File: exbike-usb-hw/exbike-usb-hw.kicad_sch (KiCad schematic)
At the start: 19 parts, among them J1 ICSP, J2 USB_B, J3 AudioJack3_SwitchTR, J4 J1, J5 J2, U1 ATtiny24A-SS, U2 AMS1117-3.3, Y1 12 MHz

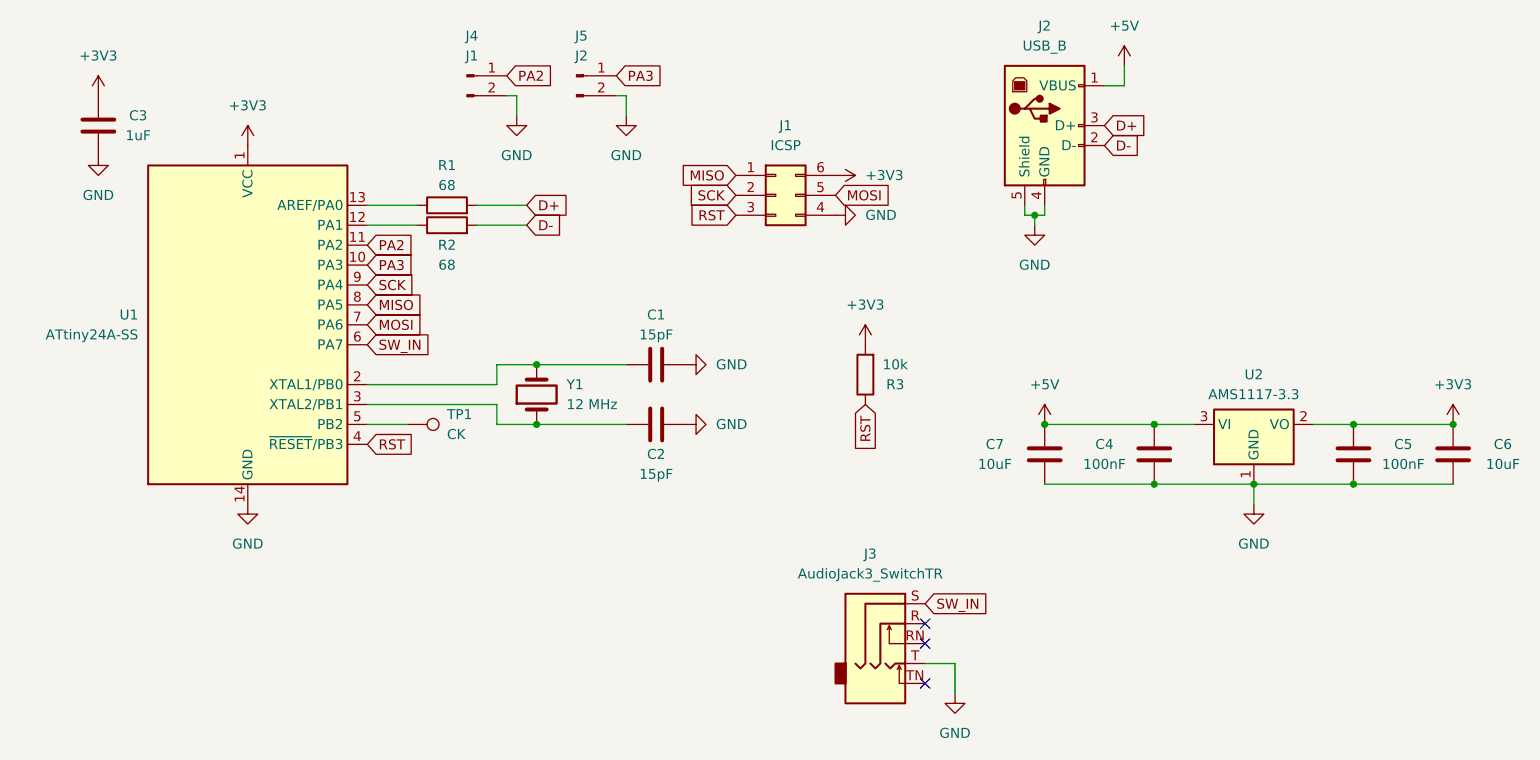
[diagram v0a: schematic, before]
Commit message: Layout
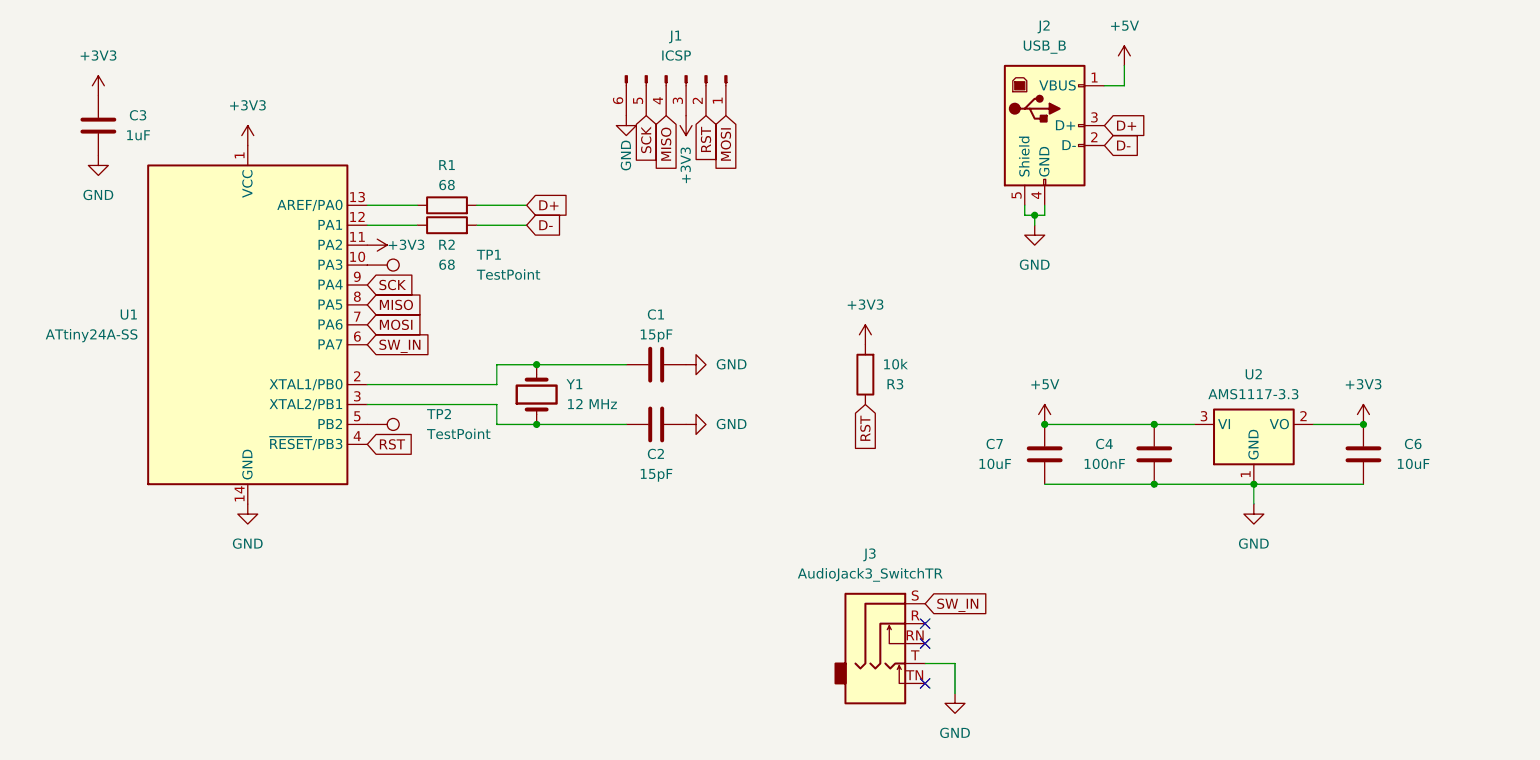
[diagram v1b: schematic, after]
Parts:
- removed C5: 100nF, Capacitor_SMD:C_0805_2012Metric_Pad1.18x1.45mm_HandSolder, symbol Device:C
- removed J1: ICSP, Connector_PinHeader_2.54mm:PinHeader_1x06_P2.54mm_Vertical, symbol Connector_Generic:Conn_02x03_Counter_Clockwise
- removed J4: J1, Connector_PinHeader_2.54mm:PinHeader_1x02_P2.54mm_Vertical, symbol Connector:Conn_01x02_Pin
- removed J5: J2, Connector_PinHeader_2.54mm:PinHeader_1x02_P2.54mm_Vertical, symbol Connector:Conn_01x02_Pin
- added J1: ICSP, Connector_PinHeader_2.54mm:PinHeader_1x06_P2.54mm_Vertical, symbol Connector:Conn_01x06_Pin
- added TP2: TestPoint, TestPoint:TestPoint_Pad_D1.0mm, symbol Connector:TestPoint
- TP1: value CK -> TestPoint; footprint TestPoint:TestPoint_Pad_1.5x1.5mm -> TestPoint:TestPoint_Pad_D1.5mm
- Y1: footprint Crystal:Crystal_SMD_3225-4Pin_3.2x2.5mm -> Crystal:Crystal_HC49-4H_Vertical
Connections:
- net PA2 is gone; now on net +3V3: U1.11 (PA2)
- net +3V3: now also J1.3 (Pin_3)
- net GND: now also J1.6 (Pin_6)
- net MISO: now also J1.4 (Pin_4)
- net MOSI: now also J1.1 (Pin_1)
- net RST: now also J1.2 (Pin_2)
- net SCK: now also J1.5 (Pin_5)
- net at C1.1, U1.2 (XTAL1/PB0): now also Y1.2; no longer Y1.3
- net at U1.5 (PB2): now also TP2.1; no longer TP1.1
- net PA3: no longer names the net of U1.10 (PA3)
- net PA3: now also TP1.1
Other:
- moved on the sheet: C6
